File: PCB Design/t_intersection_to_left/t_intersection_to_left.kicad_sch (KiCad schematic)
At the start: 8 parts, among them CN1 1X4SMT, CN2 1X4SMT, CN3 1X4SMT

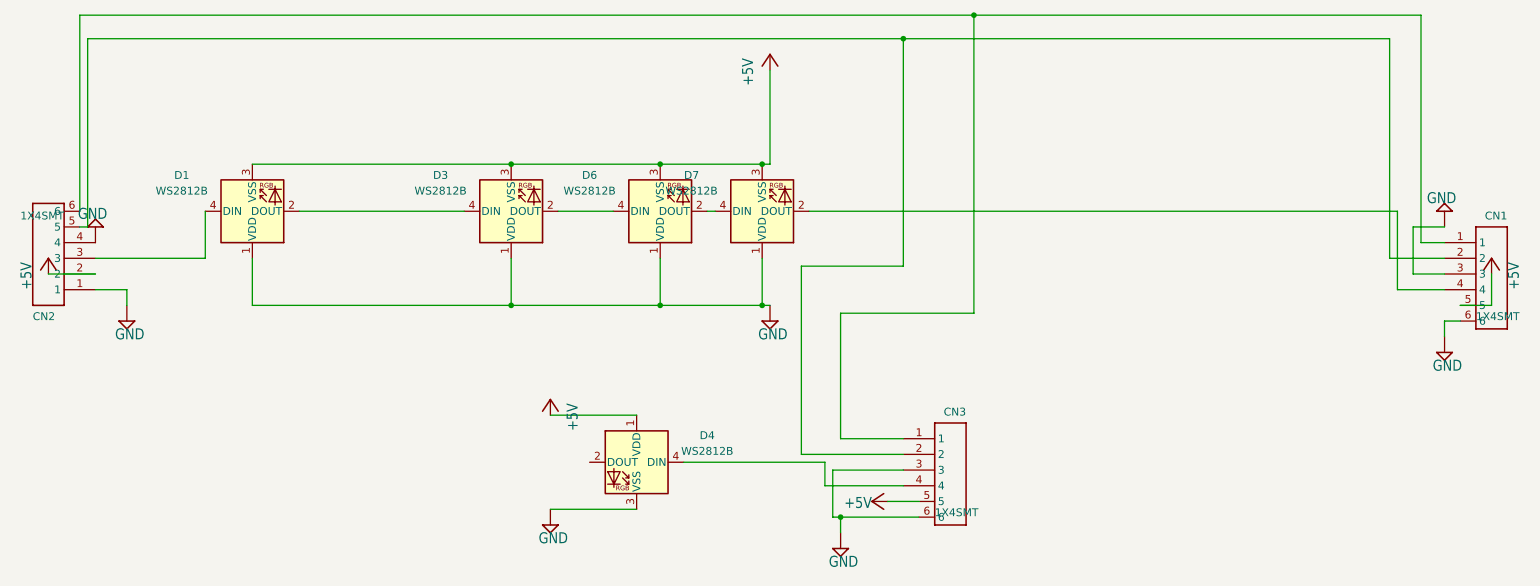
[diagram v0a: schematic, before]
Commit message: t-intersection pcbs
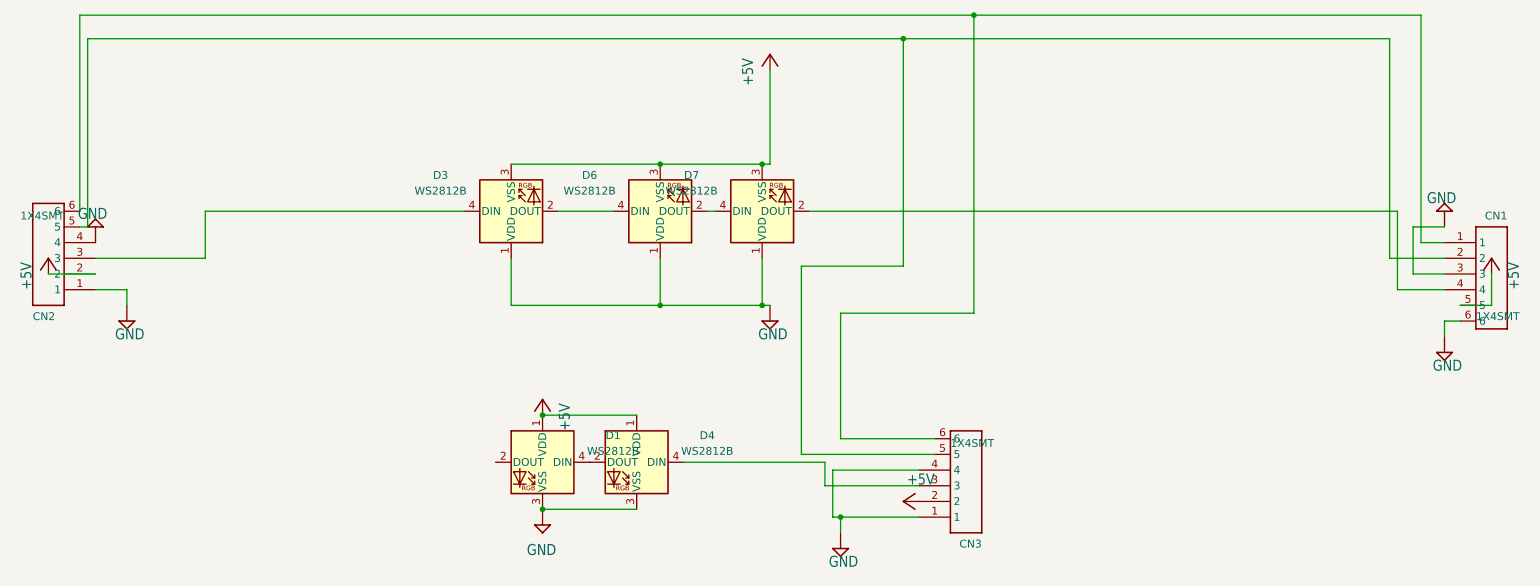
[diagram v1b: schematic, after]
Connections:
- net +5V: now also CN3.2, D1.1 (VDD); no longer CN3.5, D1.3 (VSS)
- net GND: now also CN3.1, CN3.4, D1.3 (VSS); no longer CN3.3, CN3.6, D1.1 (VDD)
- net at D4.2 (DOUT): now also D1.4 (DIN)
- net at D4.4 (DIN): now also CN3.3; no longer CN3.4
- net at CN1.1, CN2.6: now also CN3.6; no longer CN3.1
- net at CN1.2, CN2.5: now also CN3.5; no longer CN3.2
- net at D3.4 (DIN): now also CN2.3; no longer D1.2 (DOUT)
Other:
- moved on the sheet: CN3
